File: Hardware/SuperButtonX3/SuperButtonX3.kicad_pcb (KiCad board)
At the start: 2 copper layers, 123.8 x 53.2 mm, 29 parts, among them J101 USBC, J103 EXT_LED, SW101 Switch, SW102 PROG, SW103 Switch, SW104 Switch, U101 CH552G

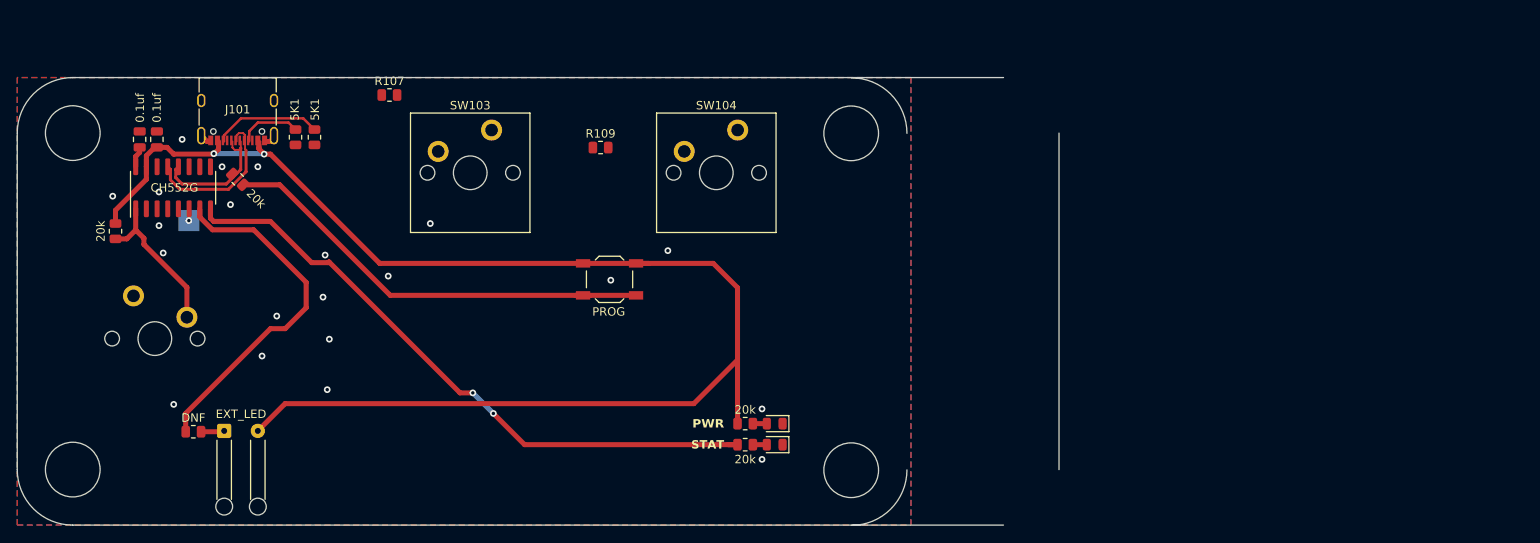
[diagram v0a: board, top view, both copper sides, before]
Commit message: Clean up x3 board
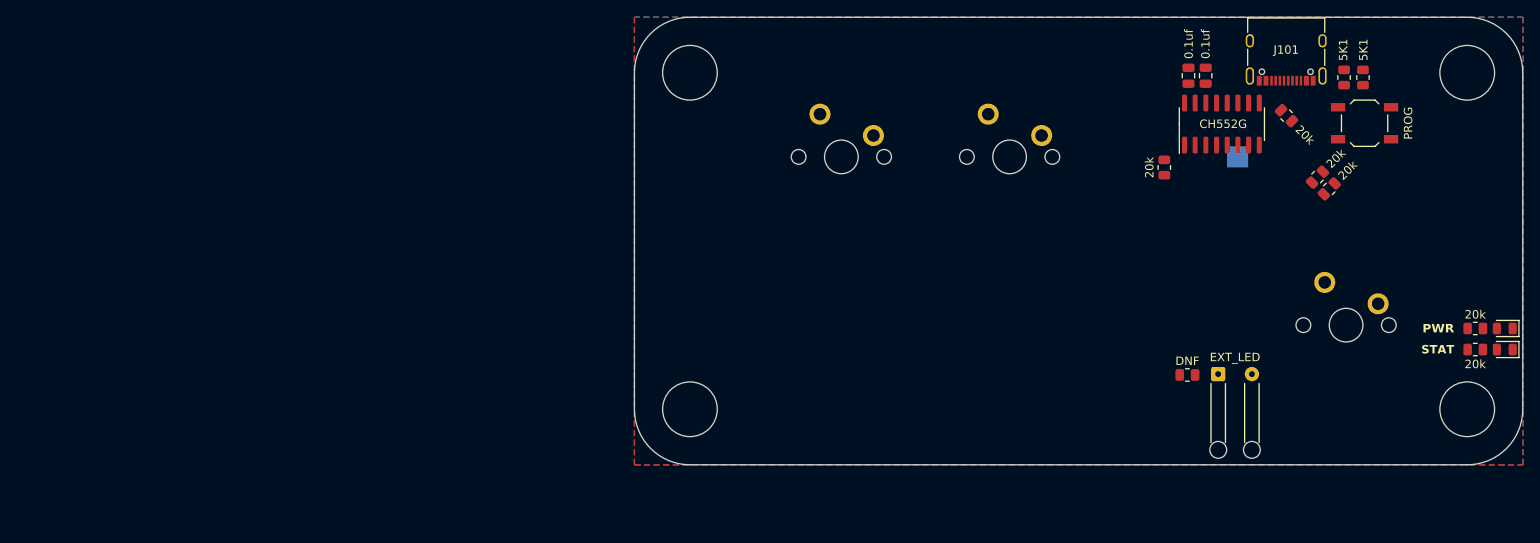
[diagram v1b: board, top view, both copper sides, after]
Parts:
- SW103, SW104: moved to B.Cu
- moved TP101 124.9 mm to (217.1, 80.0)
- moved U101 124.9 mm to (215.2, 76.1)
- moved C104 124.9 mm to (213.3, 70.3)
- moved C101 124.9 mm to (211.3, 70.3)
- moved R104 124.9 mm to (222.9, 75.1)
- moved R105 124.9 mm to (208.4, 81.3)
- moved J101 124.8 mm to (222.9, 67.3)
- moved R101 124.8 mm to (232.0, 70.6)
- moved R102 124.8 mm to (229.8, 70.6)
- moved J103 118.4 mm to (214.8, 105.8)
- moved R108 118.4 mm to (211.1, 105.9)
- moved R107 112.3 mm to (228.0, 83.8), turned to -135 degrees
- moved SW102 91.7 mm to (232.2, 76.0)
- moved D103 87.5 mm to (248.9, 102.9)
- moved D104 87.5 mm to (248.9, 100.4)
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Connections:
- U101 pad 10: unconnected-(U101-P3.3-Pad10) -> /SW_SENSE2
- U101 pad 11: unconnected-(U101-P3.4-Pad11) -> /SW_SENSE3
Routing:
- net +5V: track 170.0 -> 0.00 mm, vias 2 -> 0
- net /STAT: track 76.1 -> 0.00 mm, vias 2 -> 0
- net Net-(R104-Pad1): track 53.9 -> 0.00 mm
- net /EXT: track 41.6 -> 0.00 mm
- net /USB-: track 18.4 -> 0.00 mm
- net /SW_SENSE1: track 18.2 -> 0.00 mm
- net /USB+: track 15.8 -> 0.00 mm
- net Net-(J101-CC2): track 12.9 -> 0.00 mm
- net Net-(J101-CC1): track 7.50 -> 0.00 mm
- net Net-(J103-Pin_1): track 2.79 -> 0.00 mm
- net +3V3: track 2.49 -> 0.00 mm
- net GND: track 2.41 -> 0.00 mm, vias 21 -> 0
- net Net-(D104-A): track 1.66 -> 0.00 mm
- net Net-(D103-A): track 1.66 -> 0.00 mm
- net /RST: track 1.41 -> 0.00 mm, vias 1 -> 0
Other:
- board size 123.8 x 53.2 mm -> 105.6 x 53.2 mm
